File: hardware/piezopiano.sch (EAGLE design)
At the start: 100 parts, among them J1 CON2, Q1 DMN3404L, Q2 DMN3404L, Q3 DMN3404L, Q4 DMN3404L, Q5 DMN3404L, Q6 DMN3404L, Q7 DMN3404L, Q8 DMN3404L, Q9 DNP, U1 ATMEGA4809, U2 CH340E_MSOP10, U3 DNP

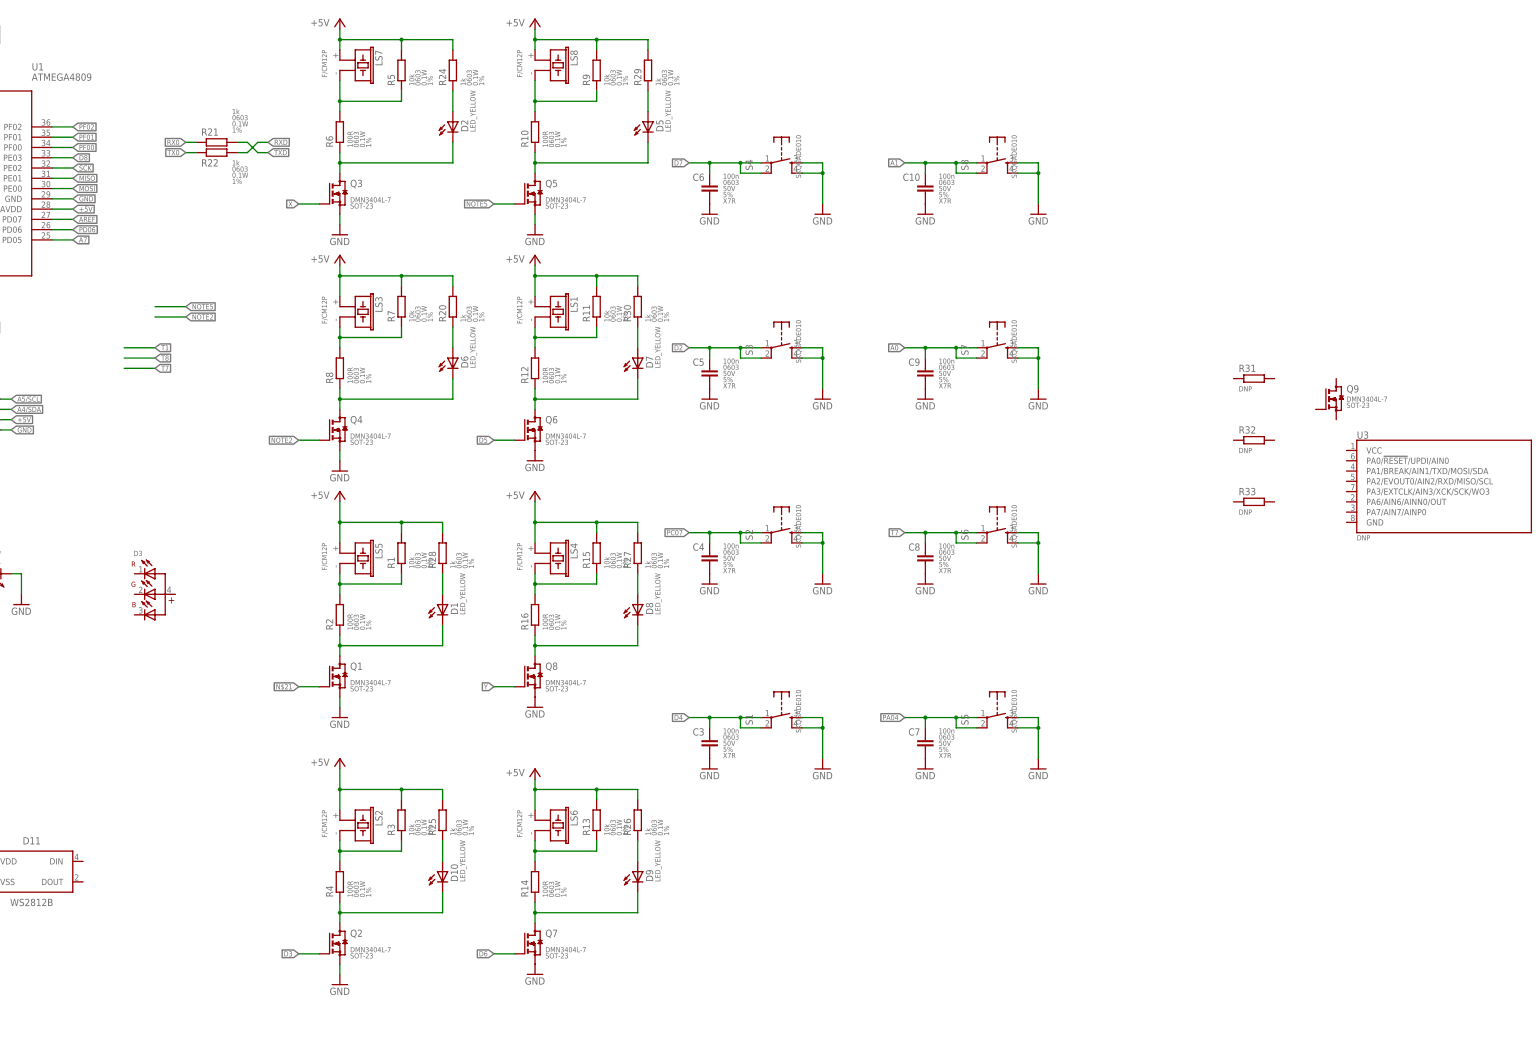
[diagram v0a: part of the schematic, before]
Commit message: Placement changes
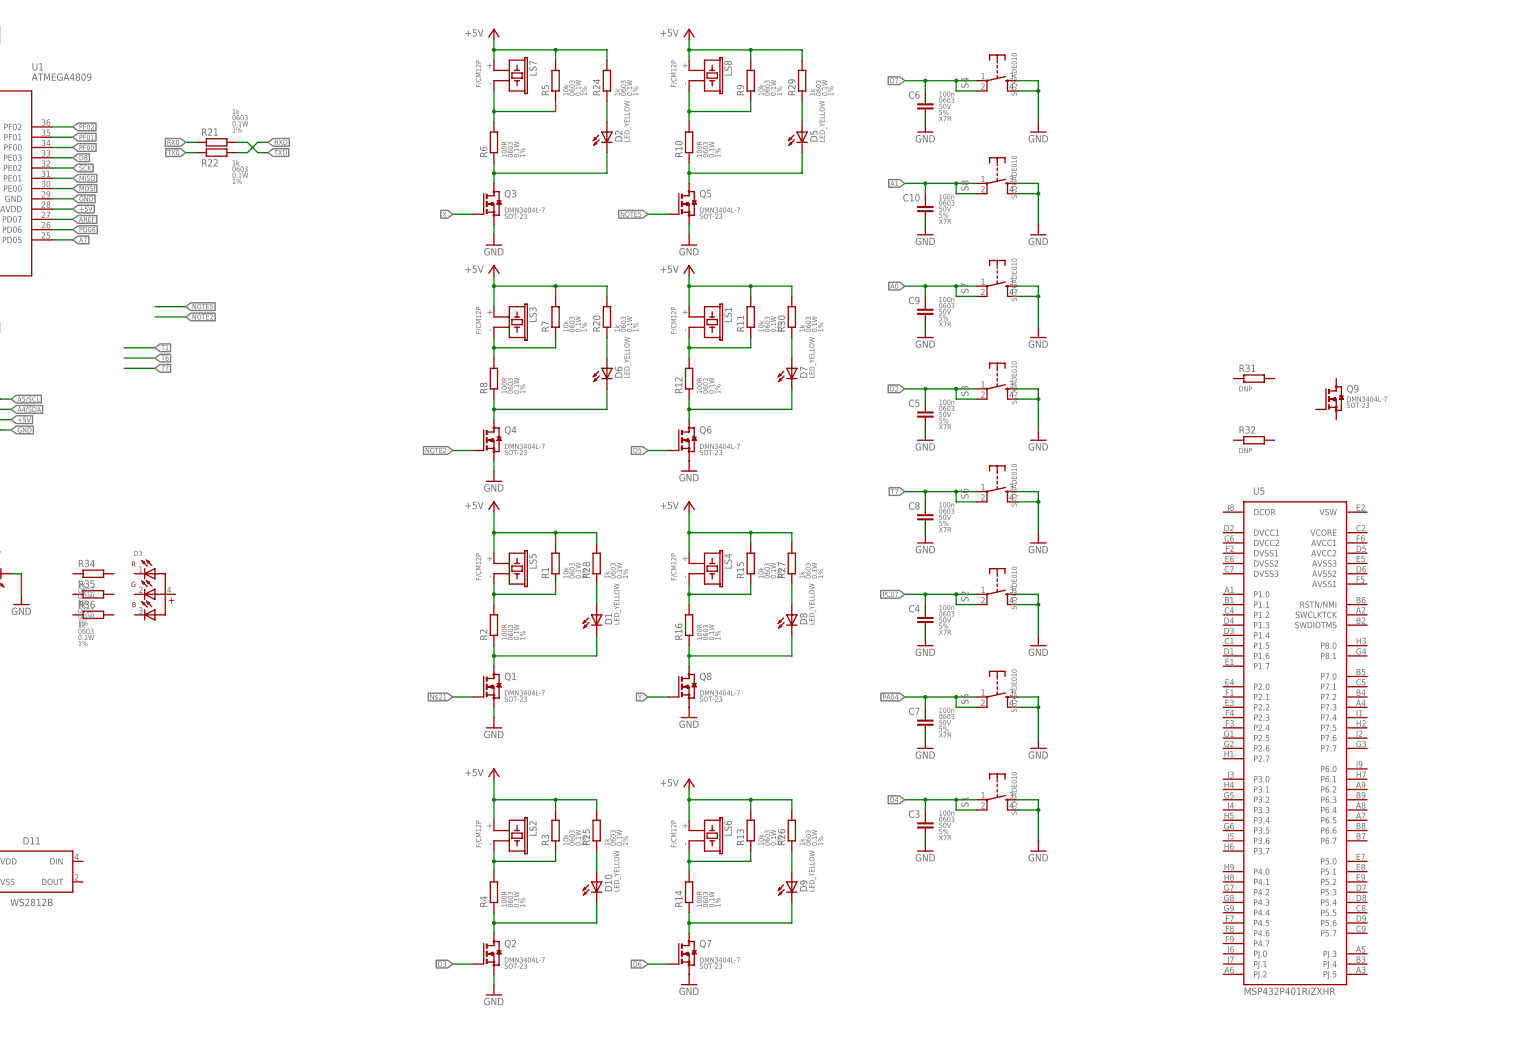
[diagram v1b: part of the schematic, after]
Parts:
- removed R33: DNP, zaan-Resistors:DNP-1206
- removed U3: DNP, zaan-IC-Microcontroller:TINY212
- added R34, R35, R36: 1k, zaan-Resistors:1KOHM-0603-1/10W-1%
- added U5: MSP432P401RIZXHR, zaan-IC-Microcontroller:MSP432P401RIZXHR
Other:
- moved on the sheet: C10, C3, C4, C5, C6, C7, C8, C9, D1, D10, D2, D5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

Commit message: Schematic cleanup
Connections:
- new net N$28: D3.R, R35.2
- new net N$35: D3.G, R34.2
- new net N$36: D3.B, R36.2
- new net N$37: R35.1
- new net N$38: R34.1
- new net N$39: R36.1
- net +5V: now also D3.4, J1.2
- net N$1: now also D11.DIN; no longer J1.2
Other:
- note added: "DNP, Size Reference"
- moved on the sheet: C11, C12, C14, C15, D11, D12, D3, D4, F1, J1, J2, J3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
